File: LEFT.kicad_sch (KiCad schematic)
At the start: 49 parts, among them Q201 2N5551, Q202 2N5401, Q203 2N5551, Q204 2N5551, Q205 2N5401, Q206 2N5401, Q207 2N5401, Q208 2N5551, Q209 MJE340, Q210 MJE340, Q211 MJE350, Q212 MJW3281, Q213 MJW1302, U101 OPA2134

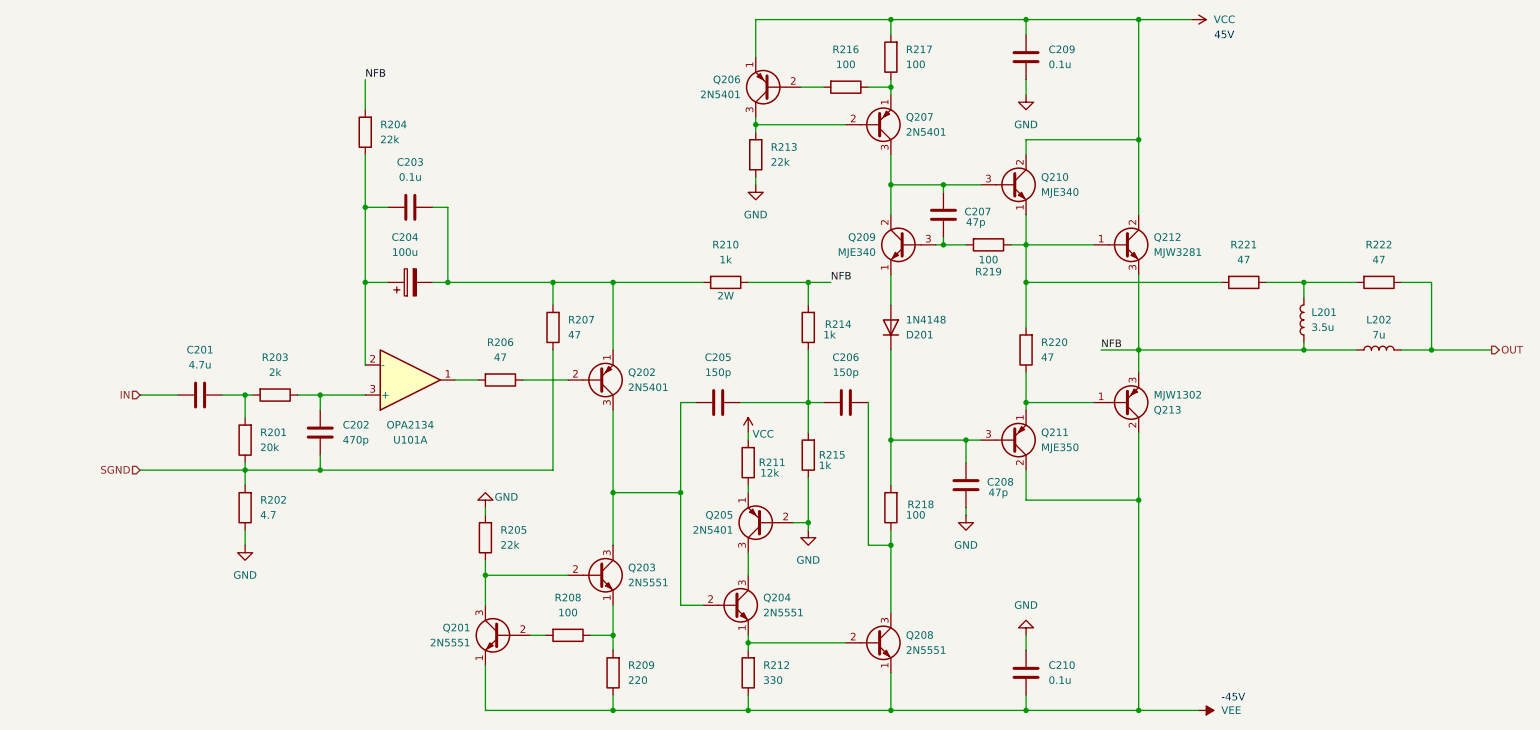
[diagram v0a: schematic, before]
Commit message: Fill attributes in schematic
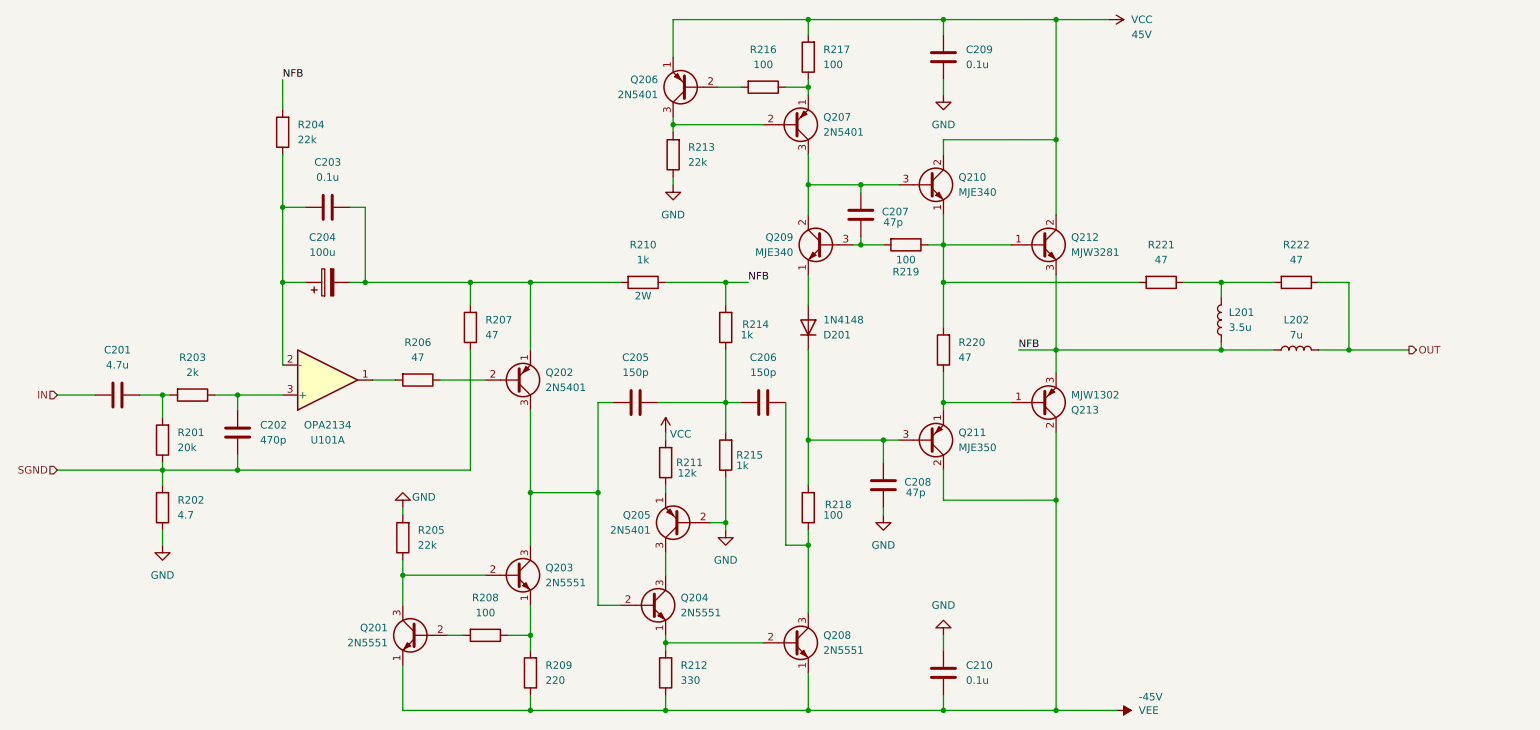
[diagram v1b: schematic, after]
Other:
- company: (none) -> jxdking
- title: (none) -> 2nd Order Current Dumping
- moved on the sheet: C201, C202, C203, C204, C205, C206, C207, C208, C209, C210, D201, L201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
